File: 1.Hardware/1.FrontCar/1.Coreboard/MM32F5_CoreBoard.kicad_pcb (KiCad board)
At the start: 4 copper layers, 47.5 x 30.9 mm, 69 parts, among them J1 IPS114, J3 BTB_02x30, J4 BTB_02x30, J5 SH1.0_4P, J7 SH1.0_2P, SW1 3x4, SW2 3x4, SW3 3x4, SW4 3x4, U1 RT9013-33GB, U3 SN65HVD232, U4 SN65HVD232, U5 MM32F5277E9P, U6 MPU-6050, Y1 32.768KHz, Y2 8MHz

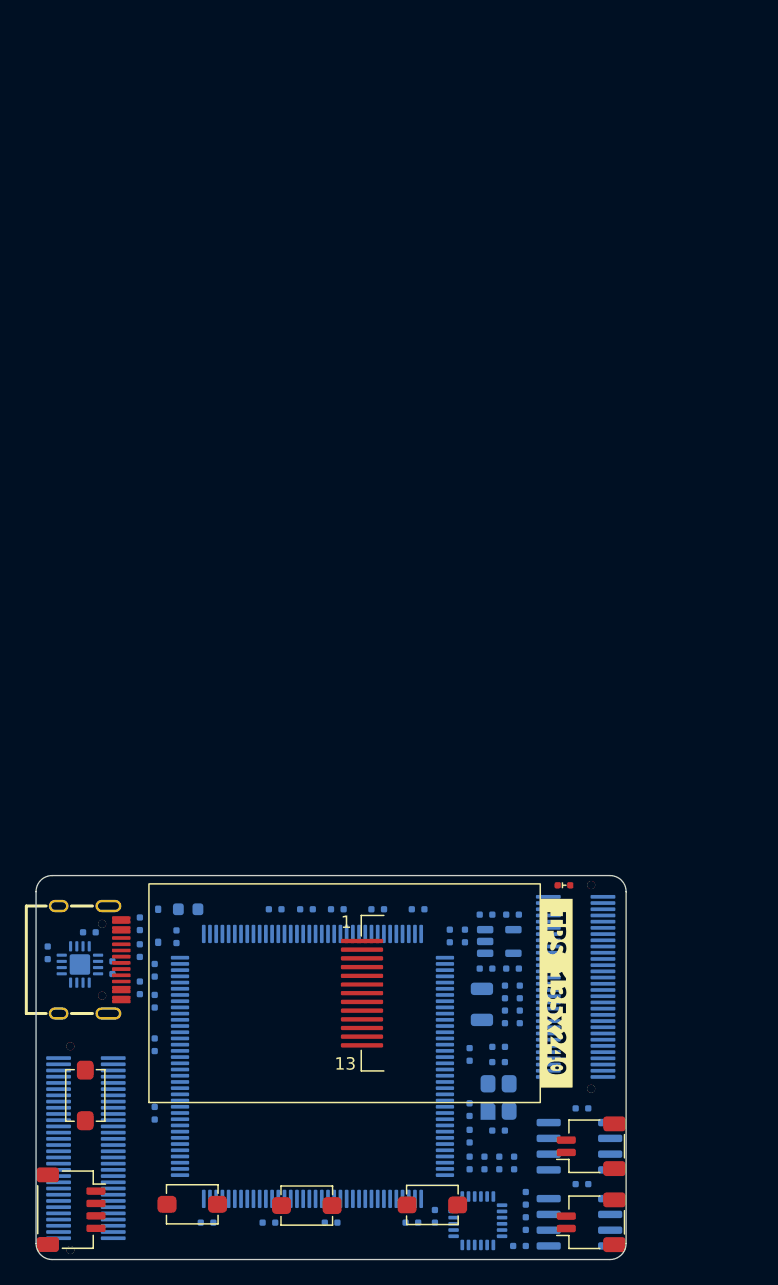
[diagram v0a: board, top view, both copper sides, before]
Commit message: 细调
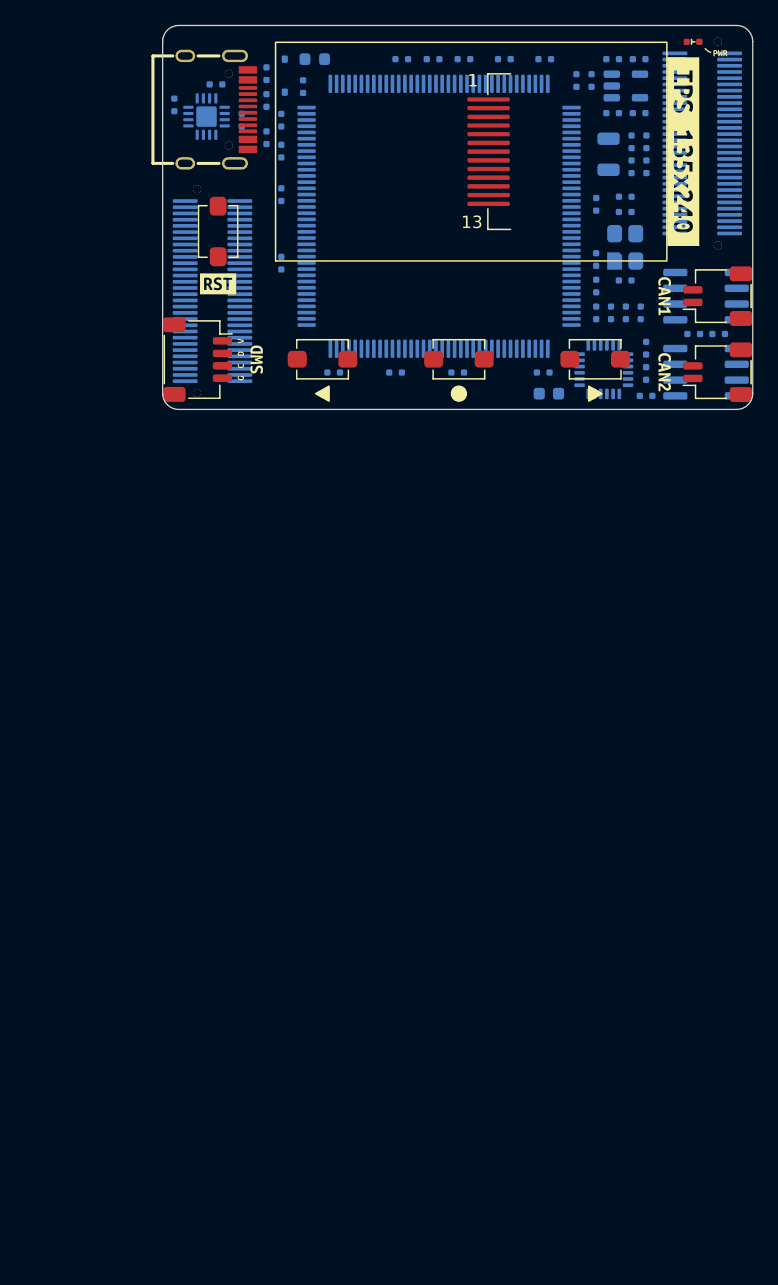
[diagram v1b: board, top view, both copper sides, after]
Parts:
- added kibuzzard-63AA82B8: G***, kibuzzard-63AA82B8, F.Cu at (80.6, 65.3)
- added kibuzzard-63AB089E: G***, kibuzzard-63AB089E, F.Cu at (83.7, 71.4)
- added kibuzzard-63AB0AE9: G***, kibuzzard-63AB0AE9, F.Cu at (82.5, 70.9)
- added kibuzzard-63AB0AFB: G***, kibuzzard-63AB0AFB, F.Cu at (82.5, 71.9)
- added kibuzzard-63AB0B00: G***, kibuzzard-63AB0B00, F.Cu at (82.5, 72.9)
- added kibuzzard-63AB0B06: G***, kibuzzard-63AB0B06, F.Cu at (82.5, 69.9)
- added kibuzzard-63AB0F85: G***, kibuzzard-63AB0F85, F.Cu at (116.6, 66.3)
- added kibuzzard-63AB0F9D: G***, kibuzzard-63AB0F9D, F.Cu at (116.6, 72.4)
- added kibuzzard-63AB10B9: G***, kibuzzard-63AB10B9, F.Cu at (121.1, 46.8)
- C30: footprint ErBW_s:C_0402 -> Capacitor_SMD:C_0603_1608Metric
- moved SW1 70.4 mm to (80.6, 61.1)
- moved J4 69.7 mm to (80.2, 65.9)
- moved C1 69.6 mm to (114.5, 51.6)
- moved C2 69.6 mm to (112.4, 51.6)
- moved C3 69.6 mm to (109.5, 49.0)
- moved C4 69.6 mm to (110.7, 49.0)
- moved C5 69.6 mm to (114.5, 47.2)
- moved R5 69.6 mm to (112.4, 47.2)
- moved U1 69.6 mm to (113.5, 49.4)
- moved SW3 69.3 mm to (111.0, 71.4)
- moved R9 69.3 mm to (120.9, 69.4)
- moved U6 69.3 mm to (111.7, 72.2)
- moved C17 69.2 mm to (106.8, 72.5)
- moved SW4 69.2 mm to (100.0, 71.4)
- moved C16 69.2 mm to (85.7, 58.1)
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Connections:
- J3 pad 1: /SWCLK -> GND
- J3 pad 10: /PD1 -> +5VA
- J3 pad 11: /PD3 -> GND
- J3 pad 12: /PG9 -> +5VA
- J3 pad 13: /PG10 -> GND
- J3 pad 14: /PG11 -> +5VA
- J3 pad 15: /PG12 -> GND
- J3 pad 16: /PG13 -> /PE2
- J3 pad 17: /PG14 -> /PE1
- J3 pad 18: /PG15 -> /PE3
- J3 pad 19: /PB3 -> /PE0
- J3 pad 2: /SWDIO -> +5VA
- J3 pad 20: /1LSB -> /PE4
- J3 pad 22: /CAN1_H -> /TOF_SCL
- J3 pad 23: /PE0 -> /1LSB
- J3 pad 24: /CAN1_L -> /TOF_SDA
- J3 pad 25: /PE2 -> /PB3
- J3 pad 26: /PE1 -> /PC13
- J3 pad 27: /PE3 -> /PG15
- J3 pad 28: /PE4 -> /PF0
- J3 pad 29: /TOF_SCL -> /PG14
- J3 pad 3: /UART1_TX -> GND
- J3 pad 30: /TOF_SDA -> /PF1
- J3 pad 31: /PC13 -> /PG13
- J3 pad 32: /PF0 -> /PF2
- J3 pad 33: /PF1 -> /PG12
- J3 pad 34: /PF2 -> /PF3
- J3 pad 35: /PF3 -> /PG11
- J3 pad 37: /PF5 -> /PG10
- J3 pad 38: /PF6 -> /PF5
- J3 pad 39: /PF7 -> /PG9
- J3 pad 4: /UART1_RX -> +5VA
- J3 pad 40: /PF8 -> /PF6
- J3 pad 41: /PF9 -> /PD3
- J3 pad 42: /PF10 -> /PF7
- J3 pad 43: /AUX_SCL -> /PD1
- J3 pad 44: /AUX_SDA -> /PF8
- J3 pad 45: /RST -> /PD0
- J3 pad 46: GND -> /PF9
- J3 pad 47: +5VA -> /PC11
- J3 pad 48: GND -> /PF10
- J3 pad 49: +5VA -> /PC10
- J3 pad 5: /SERVO -> GND
- J3 pad 50: GND -> /ADC_VBAT
- J3 pad 51: +5VA -> /SERVO
- J3 pad 52: GND -> /ADC_DIS
- J3 pad 53: +5VA -> /PH2
- J3 pad 54: GND -> /AUX_SDA
- J3 pad 55: +5VA -> /PB14
- J3 pad 56: GND -> /AUX_SCL
- J3 pad 57: +5VA -> /CAN2_H
- J3 pad 58: GND -> /CAN1_L
- J3 pad 59: +5VA -> /CAN2_L
- J3 pad 6: /PH2 -> +5VA
- J3 pad 60: GND -> /CAN1_H
- J3 pad 7: /PC11 -> GND
- J3 pad 8: /PC10 -> +5VA
- J3 pad 9: /PD0 -> GND
- J4 pad 1: /CAM_TXD -> /PB11
- J4 pad 10: /CAM_D4 -> /CAM_D0
- J4 pad 11: /CAM_D7 -> /MAPLE_CLK
- J4 pad 12: /CAM_D6 -> /CAM_D1
- J4 pad 13: /ELEMAG1 -> /MAPLE_CS
- J4 pad 14: /2PWM -> /CAM_D2
- J4 pad 15: /ELEMAG2 -> /PE10
- J4 pad 16: /2DIR -> /CAM_D3
- J4 pad 17: /ELEMAG3 -> /PE9
- J4 pad 18: /1PWM -> /CAM_D4
- J4 pad 19: /ELEMAG4 -> /PF15
- J4 pad 20: /1DIR -> /CAM_D5
- J4 pad 21: /ELEMAG5 -> /PF14
- J4 pad 22: /ADC_DIS -> /CAM_D6
- J4 pad 23: /PC5 -> /PF13
- J4 pad 24: /ADC_VBAT -> /CAM_D7
- J4 pad 25: /PB1 -> /PF12
- J4 pad 26: /PB0 -> /PB15
- J4 pad 28: /PB2-BOOT1 -> /PD8
- J4 pad 29: /PF13 -> /PB2-BOOT1
- J4 pad 3: /CAM_VSYNC -> /PB10
- J4 pad 30: /PF12 -> /PD9
- J4 pad 31: /PF15 -> /PB1
- J4 pad 32: /PF14 -> /PD10
- J4 pad 33: /PE10 -> /PB0
- J4 pad 34: /PE9 -> /PD11
- J4 pad 35: /MAPLE_CLK -> /PC5
- J4 pad 36: /MAPLE_CS -> /2LSB
- J4 pad 37: /MAPLE_MISO -> /ELEMAG5
- J4 pad 38: /CAN2_L -> /2DIR
- J4 pad 39: /MAPLE_MOSI -> /ELEMAG4
- J4 pad 4: /CAM_RXD -> /CAM_TXD
- J4 pad 40: /CAN2_H -> /PD15
- J4 pad 41: /PB10 -> /ELEMAG3
- J4 pad 42: /PE15 -> /KEY_CENTER
- J4 pad 43: /PB14 -> /ELEMAG2
- J4 pad 44: /PB11 -> /ENCODER_A
- J4 pad 45: /PD8 -> /ELEMAG1
- J4 pad 46: /PB15 -> /ENCODER_B
- J4 pad 47: /PD10 -> /2PWM
- J4 pad 48: /PD9 -> /PC8
- J4 pad 49: /2LSB -> /2DIR
- J4 pad 5: /CAM_D1 -> /PE15
- J4 pad 50: /PD11 -> /PC9
- J4 pad 51: /PD15 -> /1PWM
- J4 pad 52: /2DIR -> /PA8
- J4 pad 53: /ENCODER_A -> /1DIR
- J4 pad 54: /KEY_CENTER -> /PA9
- J4 pad 55: /PC8 -> /UART1_RX
- J4 pad 56: /ENCODER_B -> /PA10
- J4 pad 57: /PA8 -> /UART1_TX
- J4 pad 58: /PC9 -> /SWDIO
- J4 pad 59: /PA10 -> /RST
- J4 pad 6: /CAM_D0 -> /CAM_RXD
- J4 pad 60: /PA9 -> /SWCLK
- J4 pad 7: /CAM_D3 -> /MAPLE_MOSI
- J4 pad 8: /CAM_D2 -> /CAM_VSYNC
- J4 pad 9: /CAM_D5 -> /MAPLE_MISO
